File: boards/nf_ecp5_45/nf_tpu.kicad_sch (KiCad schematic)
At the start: 13 parts, among them U1 ECP5U_25_CABGA256

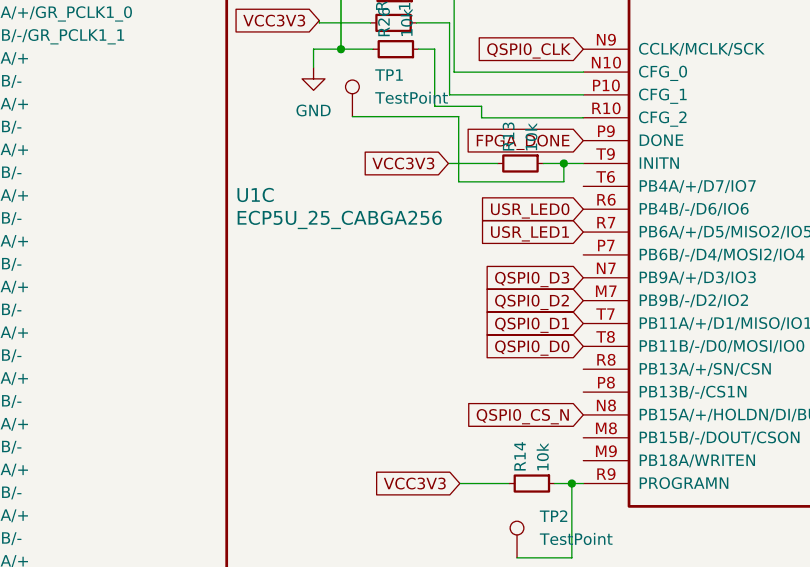
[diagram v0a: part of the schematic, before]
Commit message: board
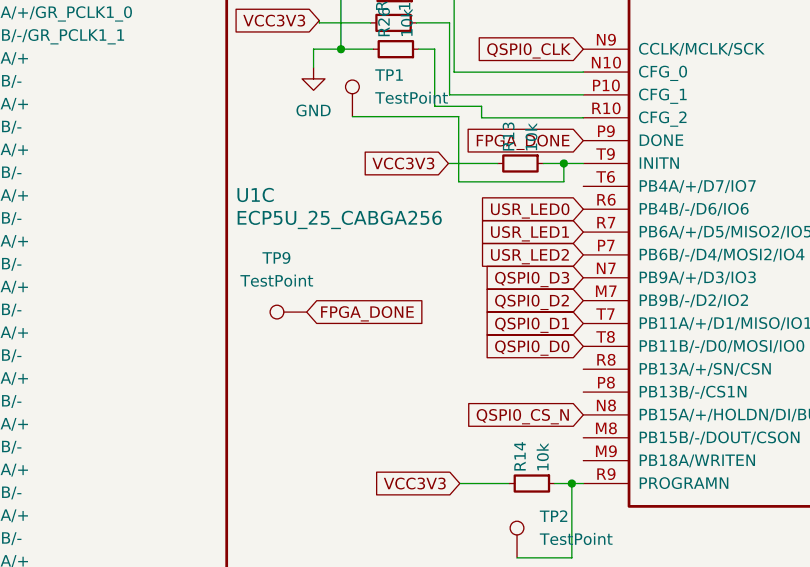
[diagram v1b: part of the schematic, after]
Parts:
- added TP9: TestPoint, TestPoint:TestPoint_Pad_D1.0mm, symbol Connector:TestPoint
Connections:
- net FPGA_DONE: now also TP9.1
- net USR_LED2: now reaches U1.P7 (PB6B/-/D4/MOSI2/IO4)
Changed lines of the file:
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@@
     (stroke (width 0) (type default))
+  )
+  (global_label "USR_LED1" (shape input) (at 179.959 94.615 180) (fields_autoplaced)
+    (effects (font (size 1.27 1.27)) (justify right))
+    (property "Intersheetrefs" "${INTERSHEET_REFS}" (at 167.5396 94.615 0)
+      (effects (font (size 1.27 1.27)) (justify right) hide)
+    )
+  )
+  (global_label "FPGA_DONE" (shape input) (at 149.225 103.505 0) (fields_autoplaced)
+    (effects (font (size 1.27 1.27)) (justify left))
+    (property "Intersheetrefs" "${INTERSHEET_REFS}" (at 162.975 103.505 0)
+      (effects (font (size 1.27 1.27)) (justify left) hide)
+    )
   )
   (global_label "VCC3V3" (shape input) (at 231.267 39.878 180) (fields_autoplaced)
@@
     )
   )
-  (global_label "USR_LED1" (shape input) (at 179.959 94.615 180) (fields_autoplaced)
-    (effects (font (size 1.27 1.27)) (justify right))
-    (property "Intersheetrefs" "${INTERSHEET_REFS}" (at 167.5396 94.615 0)
-      (effects (font (size 1.27 1.27)) (justify right) hide)
-    )
-  )
-  (global_label "USR_LED0" (shape input) (at 179.959 92.075 180) (fields_autoplaced)
-    (effects (font (size 1.27 1.27)) (justify right))
-    (property "Intersheetrefs" "${INTERSHEET_REFS}" (at 167.5396 92.075 0)
-      (effects (font (size 1.27 1.27)) (justify right) hide)
-    )
-  )
   (global_label "VCCINT" (shape input) (at 21.463 69.723 90) (fields_autoplaced)
     (effects (font (size 1.27 1.27)) (justify left))
@@
     )
   )
+  (global_label "USR_LED2" (shape input) (at 179.959 97.155 180) (fields_autoplaced)
+    (effects (font (size 1.27 1.27)) (justify right))
+    (property "Intersheetrefs" "${INTERSHEET_REFS}" (at 167.5396 97.155 0)
+      (effects (font (size 1.27 1.27)) (justify right) hide)
+    )
+  )
   (global_label "JTAG_TDO" (shape input) (at 257.937 74.93 180) (fields_autoplaced)
     (effects (font (size 1.27 1.27)) (justify right))
@@
     (effects (font (size 1.27 1.27)) (justify right))
     (property "Intersheetrefs" "${INTERSHEET_REFS}" (at 156.1216 122.555 0)
+      (effects (font (size 1.27 1.27)) (justify right) hide)
+    )
+  )
+  (global_label "USR_LED0" (shape input) (at 179.959 92.075 180) (fields_autoplaced)
+    (effects (font (size 1.27 1.27)) (justify right))
+    (property "Intersheetrefs" "${INTERSHEET_REFS}" (at 167.5396 92.075 0)
       (effects (font (size 1.27 1.27)) (justify right) hide)
     )
@@
         )
       )
+    )
+  )
+  (symbol (lib_id "Connector:TestPoint") (at 149.225 103.505 90) (unit 1)
+    (in_bom yes) (on_board yes) (dnp no) (fields_autoplaced)
+    (property "Reference" "TP9" (at 145.923 97.536 90)
+      (effects (font (size 1.27 1.27)))
+    )
+    (property "Value" "TestPoint" (at 145.923 100.076 90)
+      (effects (font (size 1.27 1.27)))
+    )
+    (property "Footprint" "TestPoint:TestPoint_Pad_D1.0mm" (at 149.225 98.425 0)
+      (effects (font (size 1.27 1.27)) hide)
+    )
+    (property "Datasheet" "~" (at 149.225 98.425 0)
+      (effects (font (size 1.27 1.27)) hide)
+    )
+    (pin "1")
+    (instances
+      (project "nf_tpu"
+        (path "/9bed7131-c603-46c6-ae3c-0e9faa418ea0"
+          (reference "TP9") (unit 1)
+        )
+      )

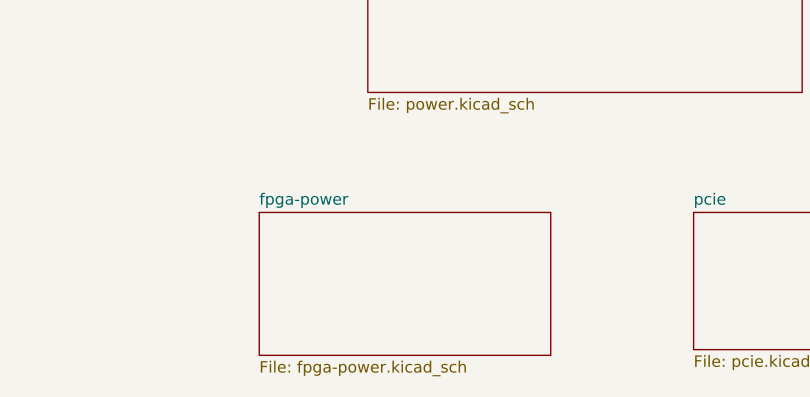
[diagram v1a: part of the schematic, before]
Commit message: schem
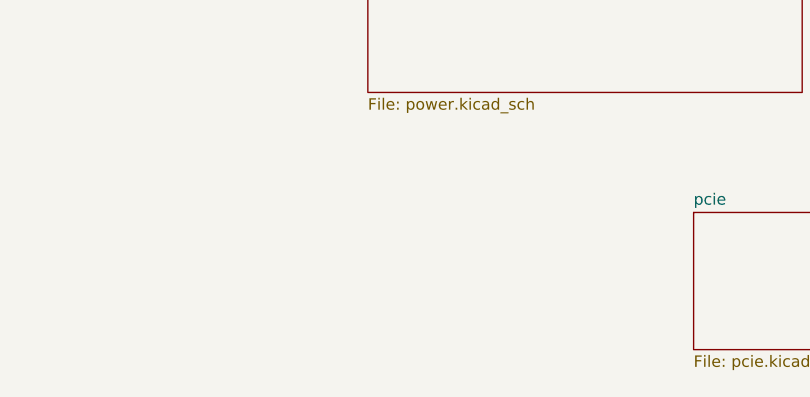
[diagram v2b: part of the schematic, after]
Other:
- removed sheet fpga-power
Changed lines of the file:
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@@
-    )
-  )
-  (sheet (at 57.023 269.621) (size 32.385 15.875) (fields_autoplaced)
-    (stroke (width 0.1524) (type solid))
-    (fill (color 0 0 0 0.0000))
-    (property "Sheetname" "fpga-power" (at 57.023 268.9094 0)
-      (effects (font (size 1.27 1.27)) (justify left bottom))
-    )
-    (property "Sheetfile" "fpga-power.kicad_sch" (at 57.023 286.0806 0)
-      (effects (font (size 1.27 1.27)) (justify left top))
-    )
-    (instances
-      (project "nf_tpu"
-        (path "/9bed7131-c603-46c6-ae3c-0e9faa418ea0" (page "7"))
-      )
     )
   )

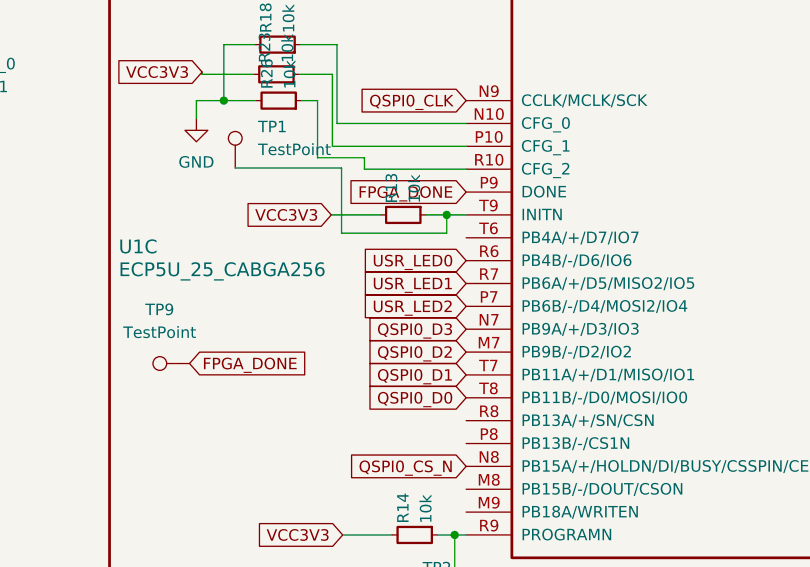
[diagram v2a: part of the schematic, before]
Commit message: board
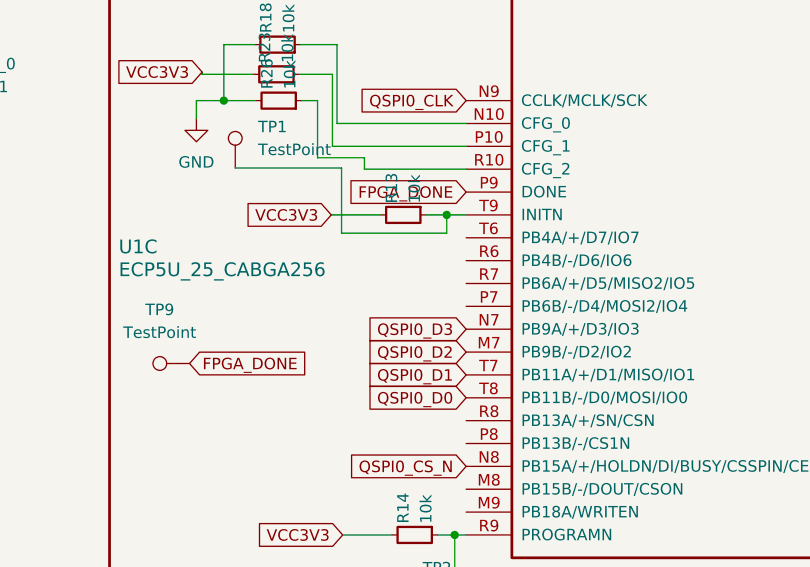
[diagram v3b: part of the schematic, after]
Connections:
- net USR_LED0: no longer names the net of U1.R6 (PB4B/-/D6/IO6)
- net USR_LED1: no longer names the net of U1.R7 (PB6A/+/D5/MISO2/IO5)
- net USR_LED2: no longer names the net of U1.P7 (PB6B/-/D4/MOSI2/IO4)
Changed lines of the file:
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@@
     (stroke (width 0) (type default))
-  )
-  (global_label "USR_LED1" (shape input) (at 179.959 94.615 180) (fields_autoplaced)
-    (effects (font (size 1.27 1.27)) (justify right))
-    (property "Intersheetrefs" "${INTERSHEET_REFS}" (at 167.5396 94.615 0)
-      (effects (font (size 1.27 1.27)) (justify right) hide)
-    )
   )
   (global_label "FPGA_DONE" (shape input) (at 149.225 103.505 0) (fields_autoplaced)
@@
     (property "Intersheetrefs" "${INTERSHEET_REFS}" (at 21.463 60.2063 90)
       (effects (font (size 1.27 1.27)) (justify left) hide)
-    )
-  )
-  (global_label "USR_LED2" (shape input) (at 179.959 97.155 180) (fields_autoplaced)
-    (effects (font (size 1.27 1.27)) (justify right))
-    (property "Intersheetrefs" "${INTERSHEET_REFS}" (at 167.5396 97.155 0)
-      (effects (font (size 1.27 1.27)) (justify right) hide)
     )
   )
@@
       (effects (font (size 1.27 1.27)) (justify right) hide)
     )
-  )
-  (global_label "USR_LED0" (shape input) (at 179.959 92.075 180) (fields_autoplaced)
-    (effects (font (size 1.27 1.27)) (justify right))
-    (property "Intersheetrefs" "${INTERSHEET_REFS}" (at 167.5396 92.075 0)
-      (effects (font (size 1.27 1.27)) (justify right) hide)
-    )
